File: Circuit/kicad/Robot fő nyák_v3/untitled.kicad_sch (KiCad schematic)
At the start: 4 parts, among them J35 Conn_01x06_Socket, J36 Conn_01x06_Socket, J37 Conn_01x06_Socket, J38 Conn_01x06_Socket

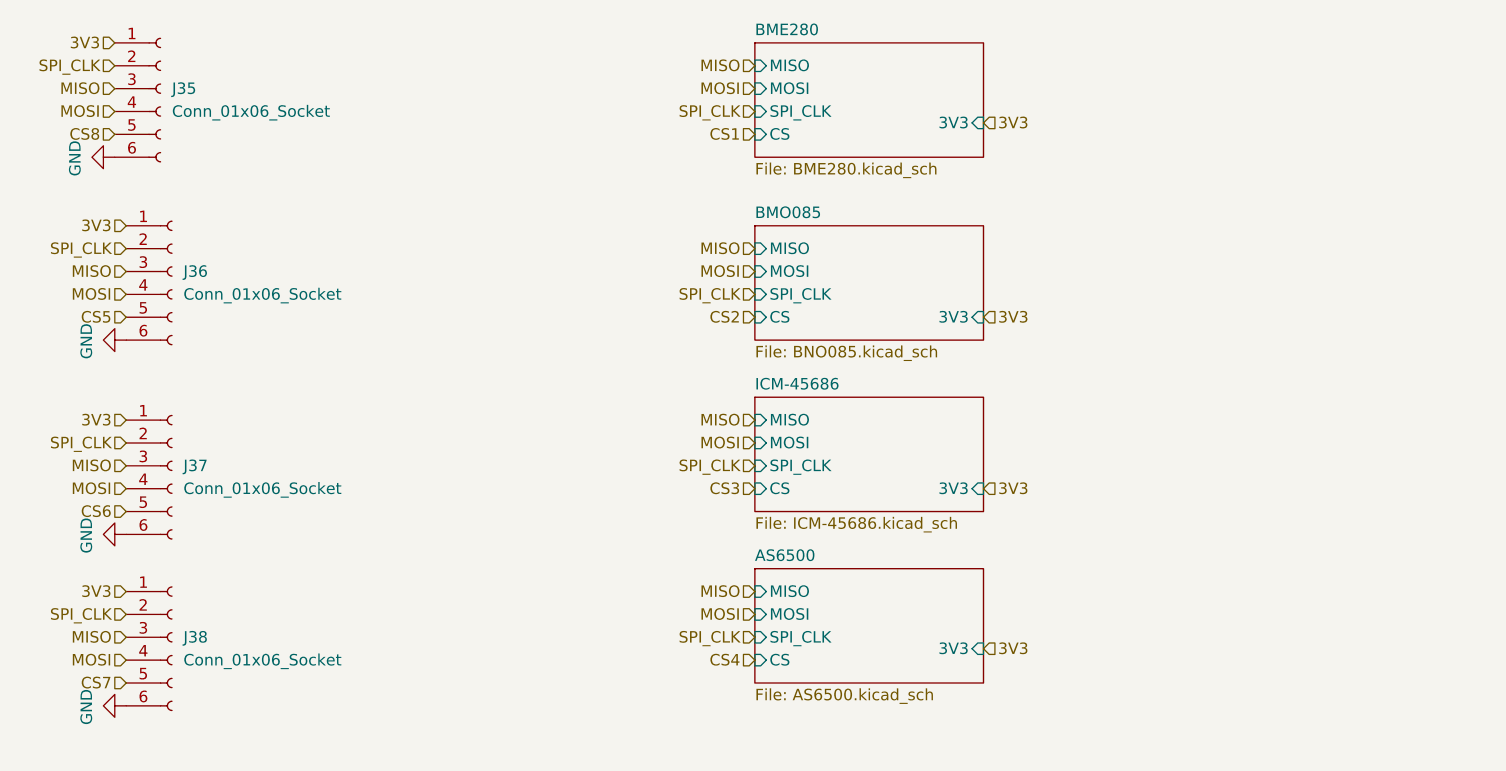
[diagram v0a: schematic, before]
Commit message: kicad update new readme media updates the circuit is 95% finished
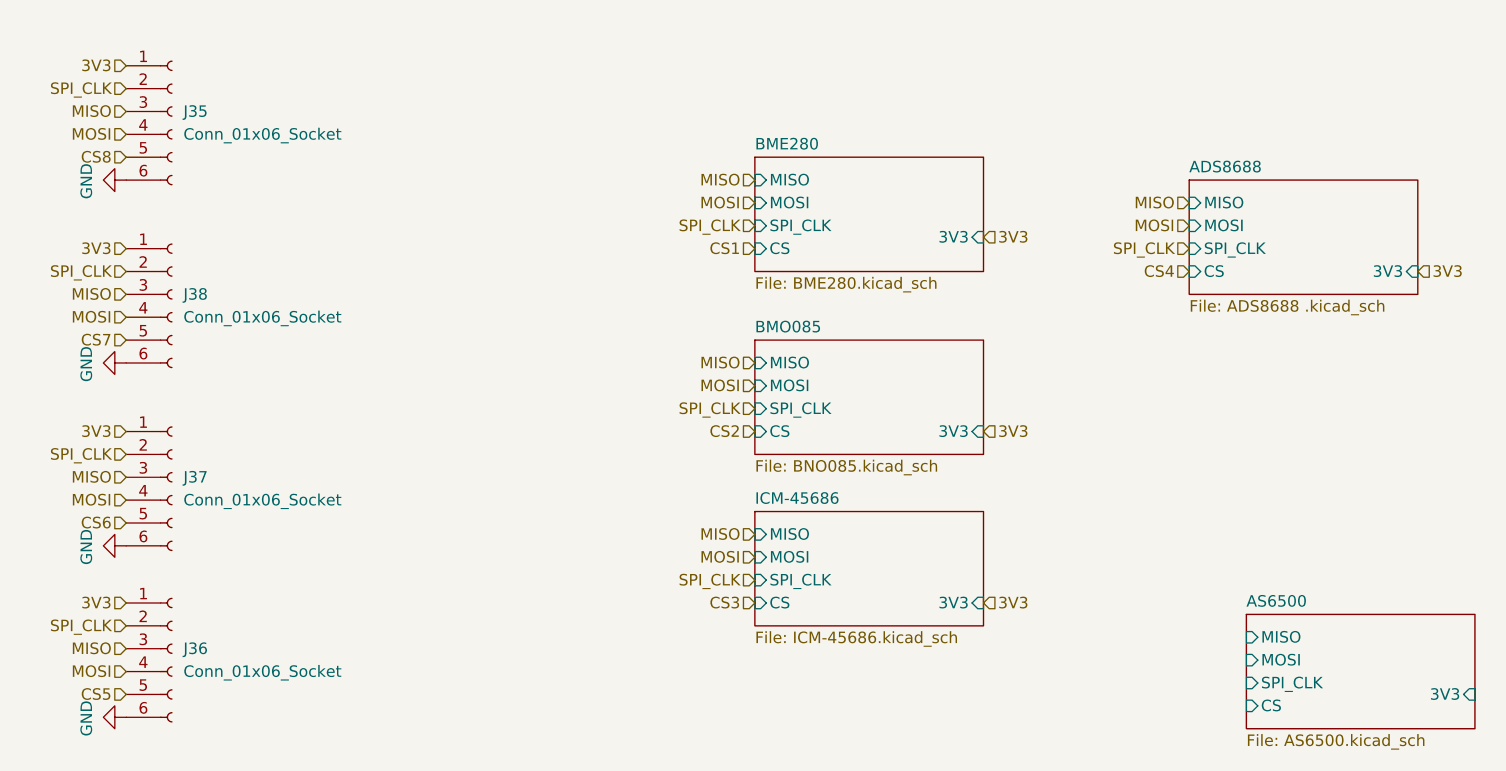
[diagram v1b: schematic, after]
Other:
- added sheet ADS8688 (ADS8688 .kicad_sch)
- moved on the sheet: J35, J36, J37, J38
